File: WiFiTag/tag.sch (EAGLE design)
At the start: 61 parts, among them IC2 MCP73831/OT

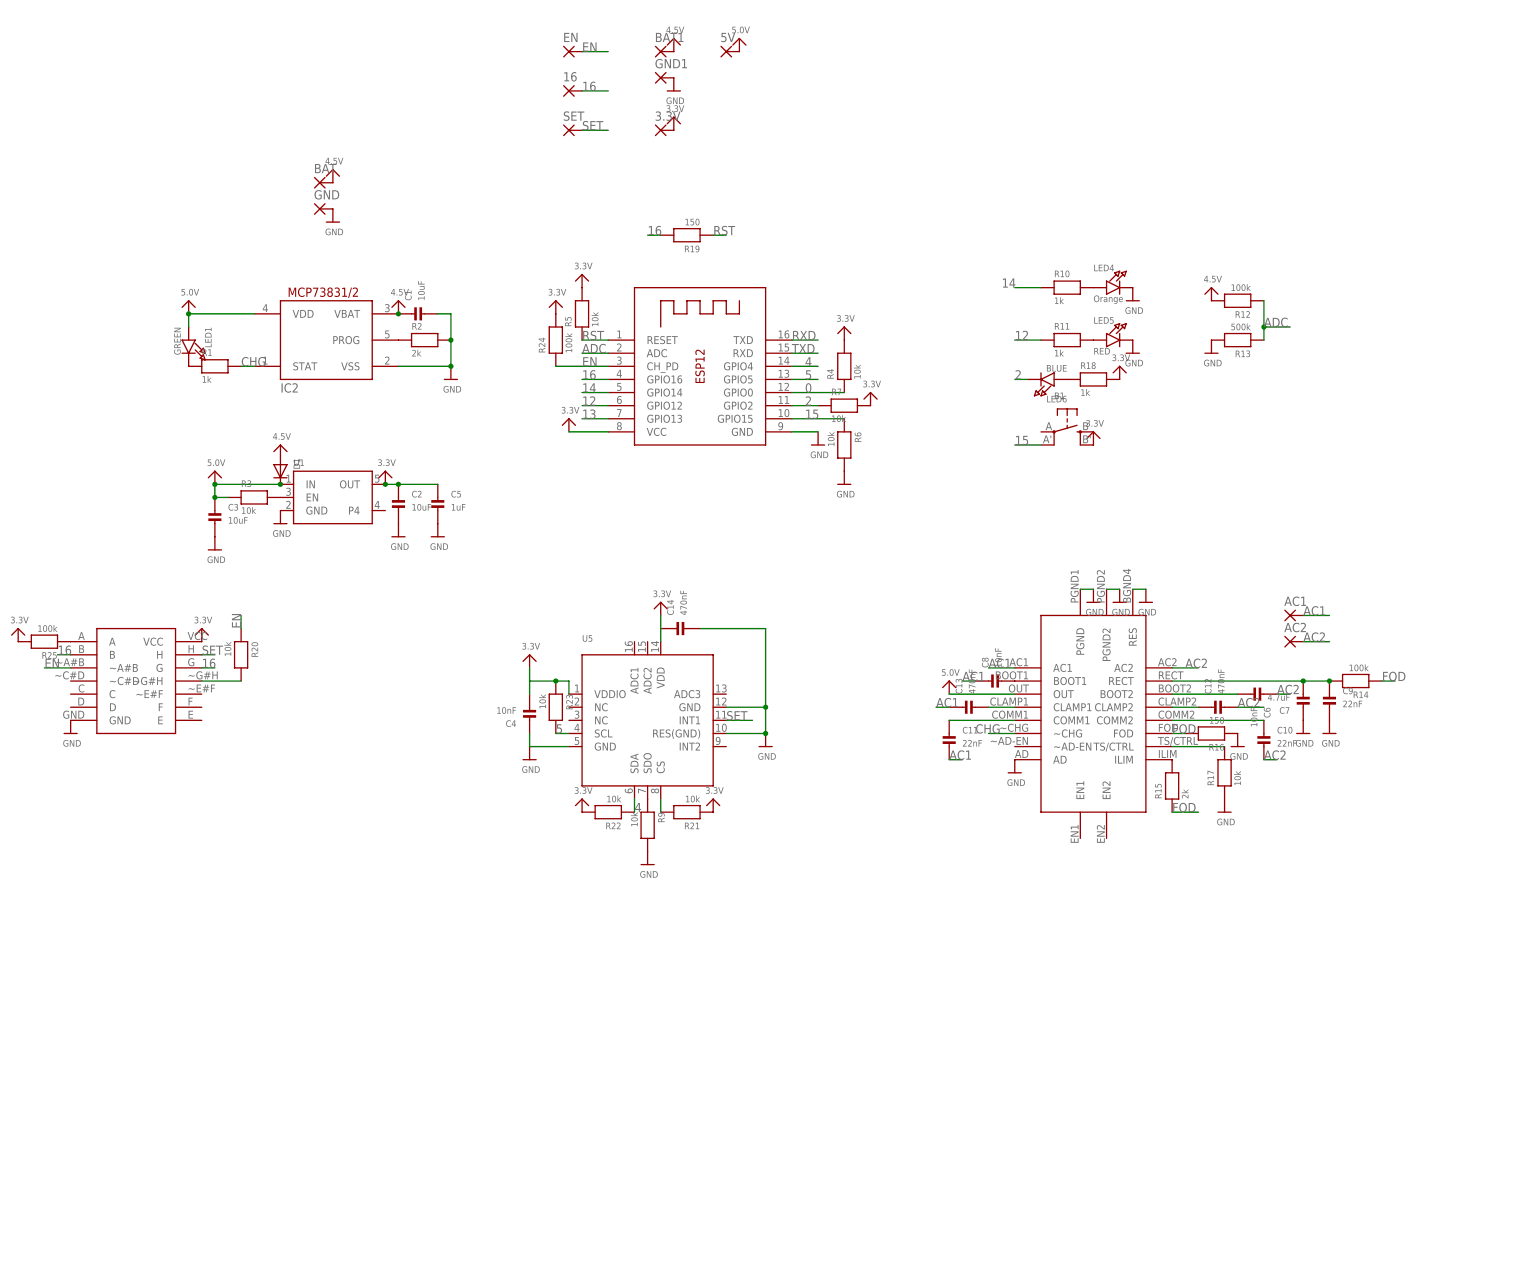
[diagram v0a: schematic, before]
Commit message: XNOR Tag version
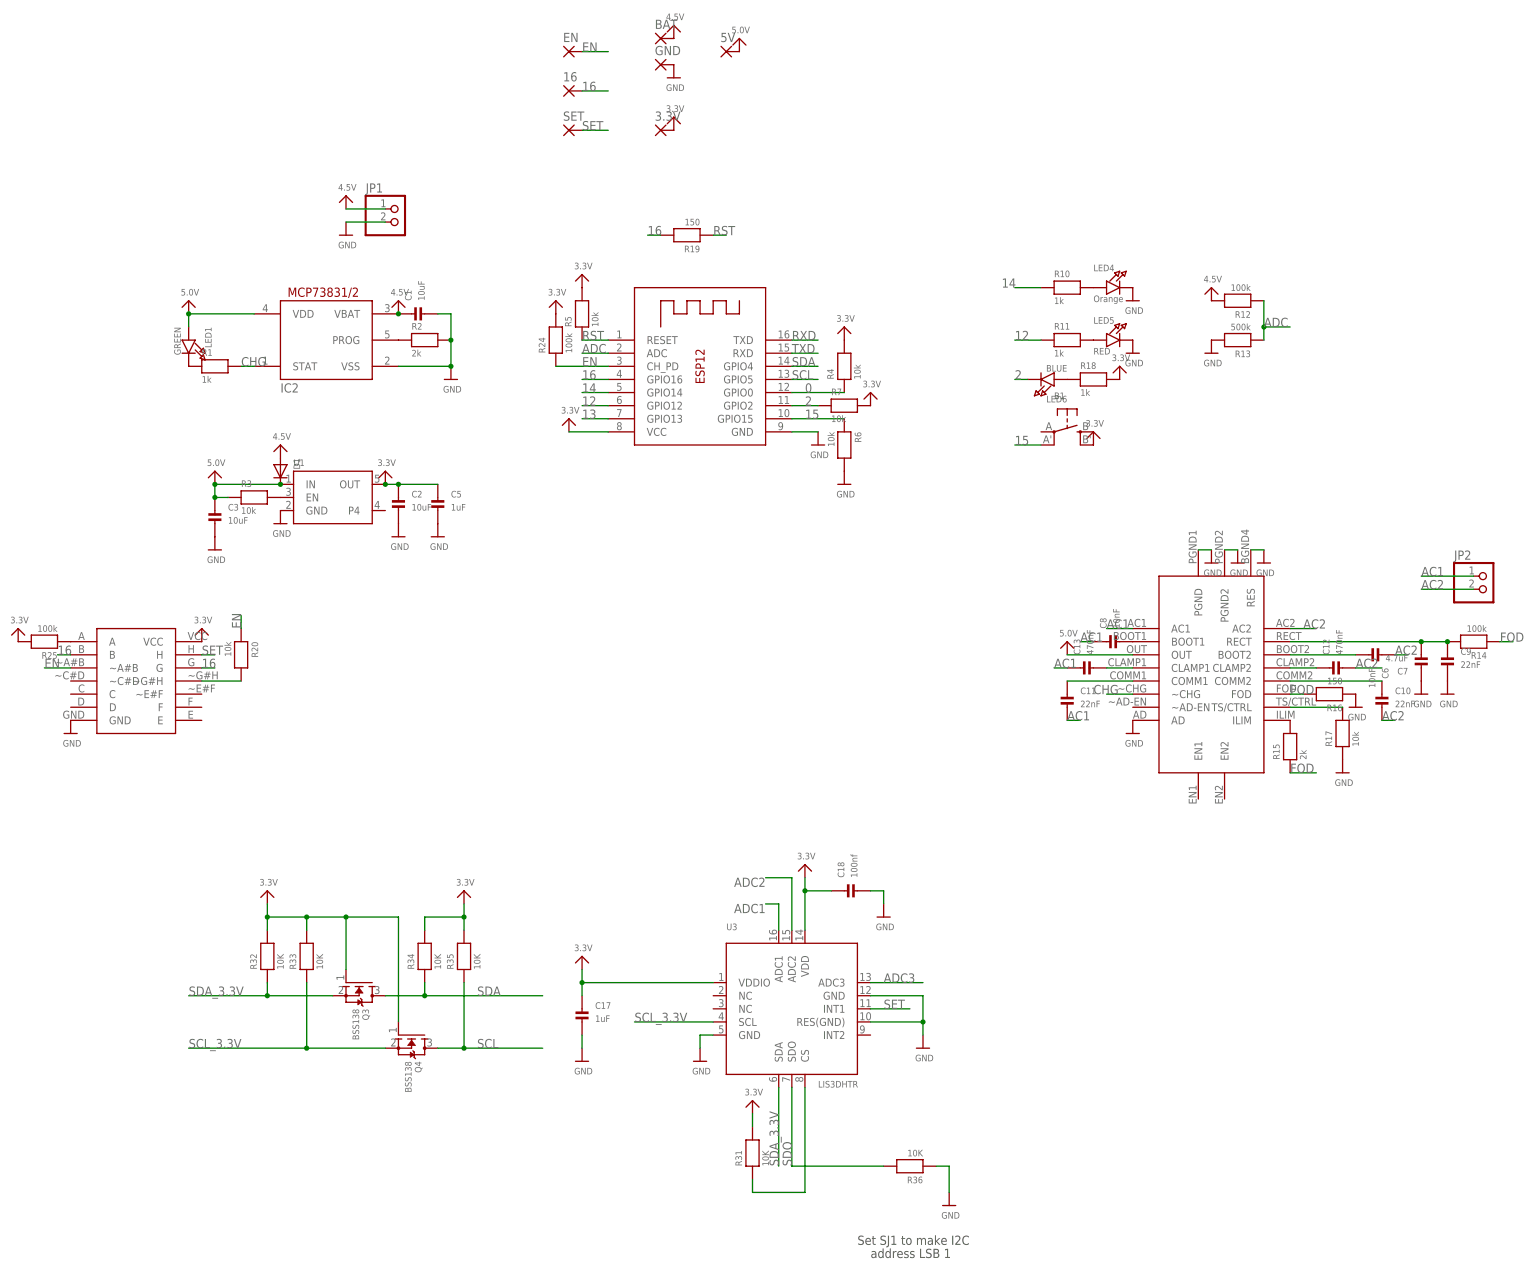
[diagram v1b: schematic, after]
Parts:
- removed AC1, AC2, BAT1, GND1: (no value), wirepad:SMD2
- removed C14: 470nF, microbuilder:CAP_CERAMIC0402
- removed C4: 10nF, microbuilder:CAP_CERAMIC0402
- removed R21, R22, R23, R9: 10k, microbuilder:RESISTOR0402
- removed U5: (no value), microbuilder:ACCEL_LIS3DHTR
- added C17: 1uF, microbuilder:CAP_CERAMIC0402
- added C18: 100nf, microbuilder:CAP_CERAMIC0402
- added JP1, JP2: (no value), microbuilder:HEADER-1X2
- added Q3, Q4: BSS138, microbuilder:MOSFET-NWIDE
- added R31, R32, R33, R34, R35, R36: 10K, microbuilder:RESISTOR0402
- added U3: LIS3DHTR, microbuilder:ACCEL_LIS3DHTR
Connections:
- removed net 4: R22.1, U5.SDA, X1.GPIO4
- removed net 5: R23.2, U5.SCL, X1.GPIO5
- removed net N$7: R9.1, U5.SDO
- removed net N$8: R21.2, U5.CS
- new net ADC1: U3.ADC1
- new net ADC2: U3.ADC2
- new net ADC3: U3.ADC3
- new net N$11: R31.1, U3.CS
- new net SCL: Q4.D, R35.1, X1.GPIO5
- new net SCL_3.3V: Q4.S, R33.1, U3.SCL
- new net SDA: Q3.D, R34.1, X1.GPIO4
- new net SDA_3.3V: Q3.S, R32.1, U3.SDA
- new net SDO: R36.2, U3.SDO
- net 3.3V: now also C17.P$1, C18.P$1, Q3.G, Q4.G, R31.2, R32.2, R33.2, R34.2, R35.2, U3.VDD, U3.VDDIO; no longer C14.P$1, C4.P$2, R21.1, R22.2, R23.1, U5.VDD, U5.VDDIO
- net 4.5V: now also JP1.1; no longer BAT1.P
- net AC1: now also JP2.1; no longer AC1.P
- net AC2: now also JP2.2; no longer AC2.P
- net GND: now also C17.P$2, C18.P$2, JP1.2, R36.1, U3.GND@1, U3.GND@2, U3.RES(GND); no longer C14.P$2, C4.P$1, GND1.P, R9.2, U5.GND@1, U5.GND@2, U5.RES(GND)
- net SET: now also U3.INT1; no longer U5.INT1
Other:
- note added: "Set SJ1 to make I2C"
- note added: "address LSB 1"
- moved on the sheet: BAT, C10, C11, C12, C13, C6, C7, C8, C9, GND, R14, R15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

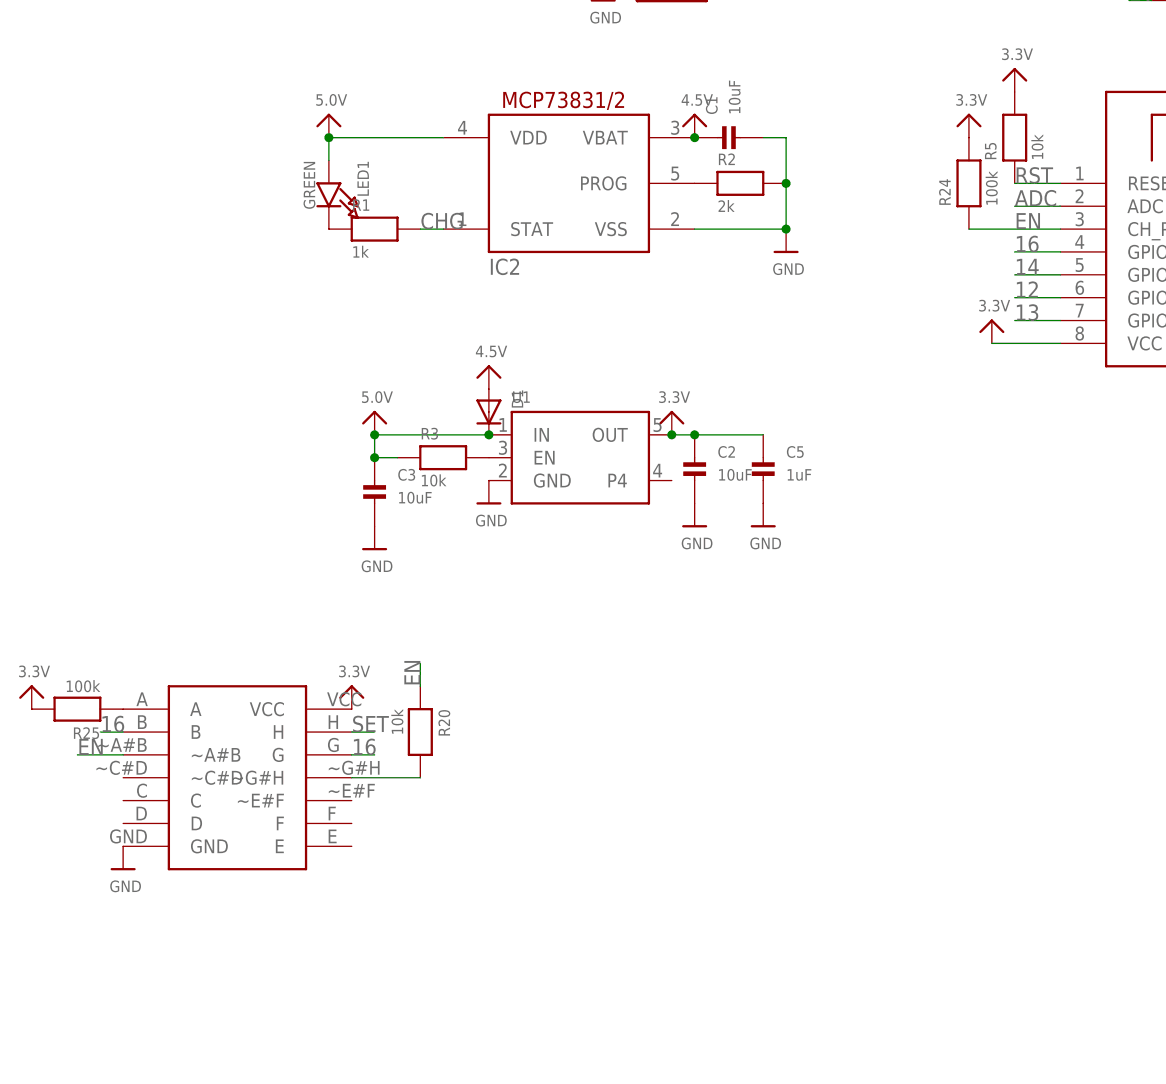
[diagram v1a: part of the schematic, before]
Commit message: V06 of PCB
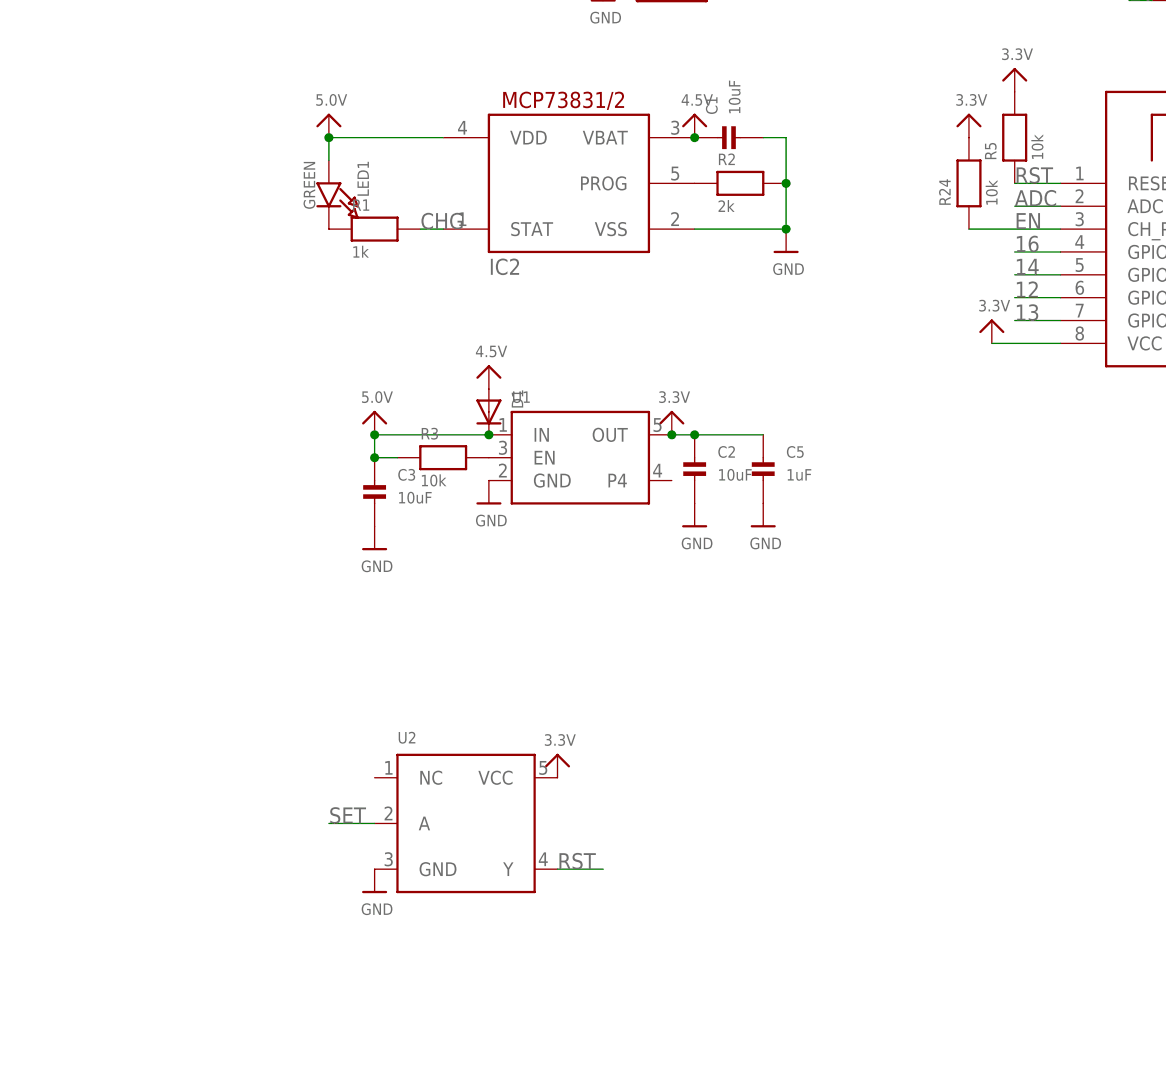
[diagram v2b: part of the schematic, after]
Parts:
- removed R20: 10k, microbuilder:RESISTOR0402
- removed R25: 100k, microbuilder:RESISTOR0402
- removed U$46: CD4077B, masterthesis:CD4077B
- added U2: (no value), microbuilder:74LVC1G04
- R24: value 100k -> 10k
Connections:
- removed net N$10: R25.1, U$46.A
- removed net N$9: R20.2, U$46.~G#H
- net 16: no longer U$46.B, U$46.G
- net 3.3V: now also U2.VCC; no longer R25.2, U$46.VCC
- net EN: no longer R20.1, U$46.~A#B
- net GND: now also U2.GND; no longer U$46.GND
- net RST: now also U2.Y
- net SET: now also U2.A; no longer U$46.H
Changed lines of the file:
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@@
 <part name="U$23" library="microbuilder" deviceset="GND" device=""/>
 <part name="U$22" library="microbuilder" deviceset="4.5V" device=""/>
-<part name="U$26" library="microbuilder" deviceset="3.3V" device=""/>
 <part name="U$31" library="microbuilder" deviceset="GND" device=""/>
 <part name="U$32" library="microbuilder" deviceset="GND" device=""/>
@@
 <part name="LED6" library="microbuilder" deviceset="LED" device="0603" value="BLUE"/>
 <part name="R19" library="microbuilder" deviceset="RESISTOR" device="0402" value="150"/>
-<part name="R20" library="microbuilder" deviceset="RESISTOR" device="0402" value="10k"/>
 <part name="R4" library="microbuilder" deviceset="RESISTOR" device="0402" value="10k"/>
 <part name="U$54" library="microbuilder" deviceset="3.3V" device=""/>
@@
 <part name="U$11" library="microbuilder" deviceset="4.5V" device=""/>
 <part name="U$14" library="microbuilder" deviceset="GND" device=""/>
-<part name="R24" library="microbuilder" deviceset="RESISTOR" device="0402" value="100k"/>
+<part name="R24" library="microbuilder" deviceset="RESISTOR" device="0402" value="10k"/>
 <part name="U$45" library="microbuilder" deviceset="3.3V" device=""/>
-<part name="U$46" library="masterthesis" deviceset="CD4077B" device=""/>
-<part name="U$47" library="microbuilder" deviceset="GND" device=""/>
-<part name="R25" library="microbuilder" deviceset="RESISTOR" device="0402" value="100k"/>
-<part name="U$48" library="microbuilder" deviceset="3.3V" device=""/>
 <part name="U3" library="microbuilder" deviceset="ACCEL_LIS3DHTR" device="" value="LIS3DHTR"/>
 <part name="U$62" library="microbuilder" deviceset="GND" device=""/>
@@
 <part name="JP1" library="microbuilder" deviceset="HEADER-1X2" device=""/>
 <part name="JP2" library="microbuilder" deviceset="HEADER-1X2" device=""/>
+<part name="U2" library="microbuilder" deviceset="74LVC1G04" device=""/>
+<part name="U$24" library="microbuilder" deviceset="3.3V" device=""/>
+<part name="U$25" library="microbuilder" deviceset="GND" device=""/>
 </parts>
 <sheets>
@@
 <instance part="U$23" gate="G$1" x="111.76" y="17.78"/>
 <instance part="U$22" gate="G$1" x="111.76" y="30.48"/>
-<instance part="U$26" gate="G$1" x="-83.82" y="-35.56"/>
 <instance part="U$31" gate="G$1" x="121.92" y="-22.86"/>
 <instance part="U$32" gate="G$1" x="116.84" y="-22.86"/>
@@
 <instance part="LED6" gate="G$1" x="78.74" y="12.7" rot="R180"/>
 <instance part="R19" gate="G$1" x="10.16" y="40.64" rot="R180"/>
-<instance part="R20" gate="G$1" x="-76.2" y="-40.64" rot="R270"/>
 <instance part="R4" gate="G$1" x="40.64" y="15.24" rot="R90"/>
 <instance part="U$54" gate="G$1" x="40.64" y="22.86"/>
@@
 <instance part="R24" gate="G$1" x="-15.24" y="20.32" rot="R90"/>
 <instance part="U$45" gate="G$1" x="-15.24" y="27.94"/>
-<instance part="U$46" gate="G$1" x="-96.52" y="-45.72"/>
-<instance part="U$47" gate="G$1" x="-109.22" y="-55.88"/>
-<instance part="R25" gate="G$1" x="-114.3" y="-38.1" rot="R180"/>
-<instance part="U$48" gate="G$1" x="-119.38" y="-35.56"/>
 <instance part="U3" gate="G$1" x="30.48" y="-109.22"/>
 <instance part="U$62" gate="G$1" x="12.7" y="-119.38"/>
@@
 <instance part="JP1" gate="G$1" x="-45.72" y="43.18"/>
 <instance part="JP2" gate="G$1" x="165.1" y="-27.94"/>
+<instance part="U2" gate="G$1" x="-71.12" y="-50.8"/>
+<instance part="U$24" gate="G$1" x="-60.96" y="-43.18"/>
+<instance part="U$25" gate="G$1" x="-81.28" y="-58.42"/>
 </instances>
 <busses>
@@
 </segment>
 <segment>
-<pinref part="U$46" gate="G$1" pin="GND"/>
-<pinref part="U$47" gate="G$1" pin="GND"/>
-</segment>
-<segment>
 <pinref part="U3" gate="G$1" pin="GND@1"/>
 <pinref part="U$62" gate="G$1" pin="GND"/>
@@
 <wire x1="-55.88" y1="43.18" x2="-48.26" y2="43.18" width="0.1524" layer="91"/>
 </segment>
+<segment>
+<pinref part="U2" gate="G$1" pin="GND"/>
+<pinref part="U$25" gate="G$1" pin="GND"/>
+</segment>
 </net>
 <net name="3.3V" class="0">
@@
 <pinref part="R24" gate="G$1" pin="2"/>
 <pinref part="U$45" gate="G$1" pin="3.3V"/>
-</segment>
-<segment>
-<pinref part="U$46" gate="G$1" pin="VCC"/>
-<pinref part="U$26" gate="G$1" pin="3.3V"/>
-</segment>
-<segment>
-<pinref part="R25" gate="G$1" pin="2"/>
-<pinref part="U$48" gate="G$1" pin="3.3V"/>
 </segment>
 <segment>
@@
 <pinref part="U$21" gate="G$1" pin="3.3V"/>
 </segment>
+<segment>
+<pinref part="U2" gate="G$1" pin="VCC"/>
+<pinref part="U$24" gate="G$1" pin="3.3V"/>
+</segment>
 </net>
 <net name="N$5" class="0">
@@
 </segment>
 <segment>
-<pinref part="U$46" gate="G$1" pin="H"/>
-<wire x1="-83.82" y1="-40.64" x2="-81.28" y2="-40.64" width="0.1524" layer="91"/>
-<label x="-83.82" y="-40.64" size="1.778" layer="95"/>
-</segment>
-<segment>
 <pinref part="U3" gate="G$1" pin="INT1"/>
 <wire x1="45.72" y1="-109.22" x2="53.34" y2="-109.22" width="0.1524" layer="91"/>
 <label x="48.26" y="-109.22" size="1.778" layer="95"/>
+</segment>
+<segment>
+<pinref part="U2" gate="G$1" pin="A"/>
+<wire x1="-81.28" y1="-50.8" x2="-86.36" y2="-50.8" width="0.1524" layer="91"/>
+<label x="-86.36" y="-50.8" size="1.778" layer="95"/>
 </segment>
 </net>
@@
 <label x="15.24" y="40.64" size="1.778" layer="95"/>
 <pinref part="R19" gate="G$1" pin="1"/>
+</segment>
+<segment>
+<pinref part="U2" gate="G$1" pin="Y"/>
+<wire x1="-60.96" y1="-55.88" x2="-55.88" y2="-55.88" width="0.1524" layer="91"/>
+<label x="-60.96" y="-55.88" size="1.778" layer="95"/>
 </segment>
 </net>
@@
 <label x="-10.16" y="76.2" size="1.778" layer="95"/>
 </segment>
-<segment>
-<pinref part="R20" gate="G$1" pin="1"/>
-<wire x1="-76.2" y1="-35.56" x2="-76.2" y2="-33.02" width="0.1524" layer="91"/>
-<label x="-76.2" y="-35.56" size="1.778" layer="95" rot="R90"/>
-</segment>
-<segment>
-<pinref part="U$46" gate="G$1" pin="~A#B"/>
-<wire x1="-109.22" y1="-43.18" x2="-114.3" y2="-43.18" width="0.1524" layer="91"/>
-<label x="-114.3" y="-43.18" size="1.778" layer="95"/>
-</segment>
 </net>
 <net name="16" class="0">
@@
 <wire x1="-10.16" y1="68.58" x2="-5.08" y2="68.58" width="0.1524" layer="91"/>
 <label x="-10.16" y="68.58" size="1.778" layer="95"/>
-</segment>
-<segment>
-<pinref part="U$46" gate="G$1" pin="G"/>
-<wire x1="-83.82" y1="-43.18" x2="-81.28" y2="-43.18" width="0.1524" layer="91"/>
-<label x="-83.82" y="-43.18" size="1.778" layer="95"/>
-</segment>
-<segment>
-<pinref part="U$46" gate="G$1" pin="B"/>
-<wire x1="-109.22" y1="-40.64" x2="-111.76" y2="-40.64" width="0.1524" layer="91"/>
-<label x="-111.76" y="-40.64" size="1.778" layer="95"/>
 </segment>
 </net>
@@
 </segment>
 </net>
-<net name="N$9" class="0">
-<segment>
-<pinref part="U$46" gate="G$1" pin="~G#H"/>
-<pinref part="R20" gate="G$1" pin="2"/>
-<wire x1="-76.2" y1="-45.72" x2="-83.82" y2="-45.72" width="0.1524" layer="91"/>
-</segment>
-</net>
-<net name="N$10" class="0">
-<segment>
-<pinref part="U$46" gate="G$1" pin="A"/>
-<pinref part="R25" gate="G$1" pin="1"/>
-</segment>
-</net>
